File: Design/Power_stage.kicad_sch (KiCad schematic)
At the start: 25 parts, among them IC4 LM60440ARPKR, U3 CRE1S0505S3C, U6 CRE1S0505S3C, U8 LP3963-3.3

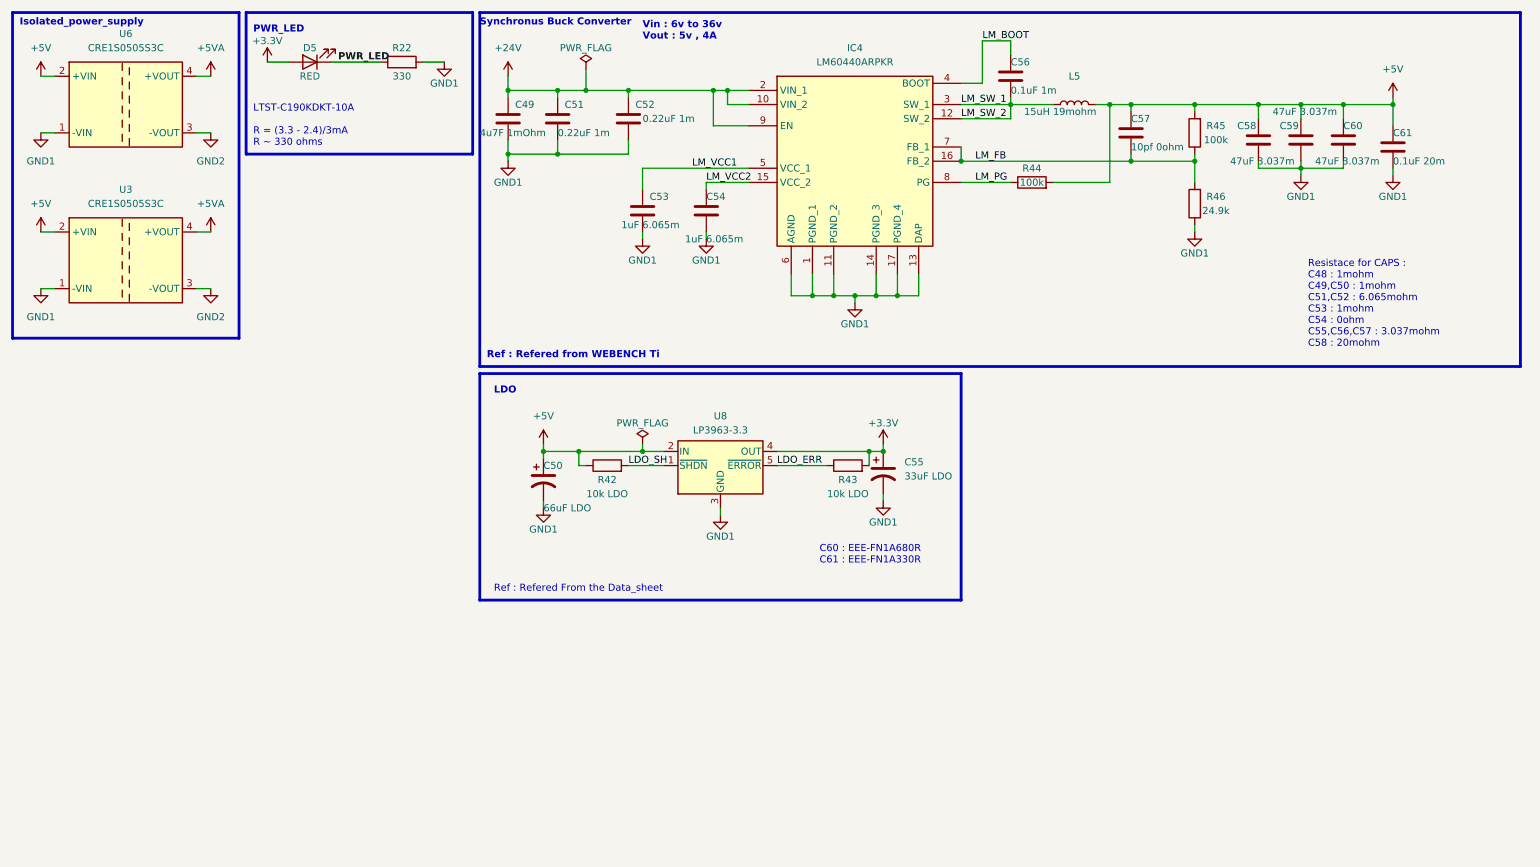
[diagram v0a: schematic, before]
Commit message: Schematic Design complete
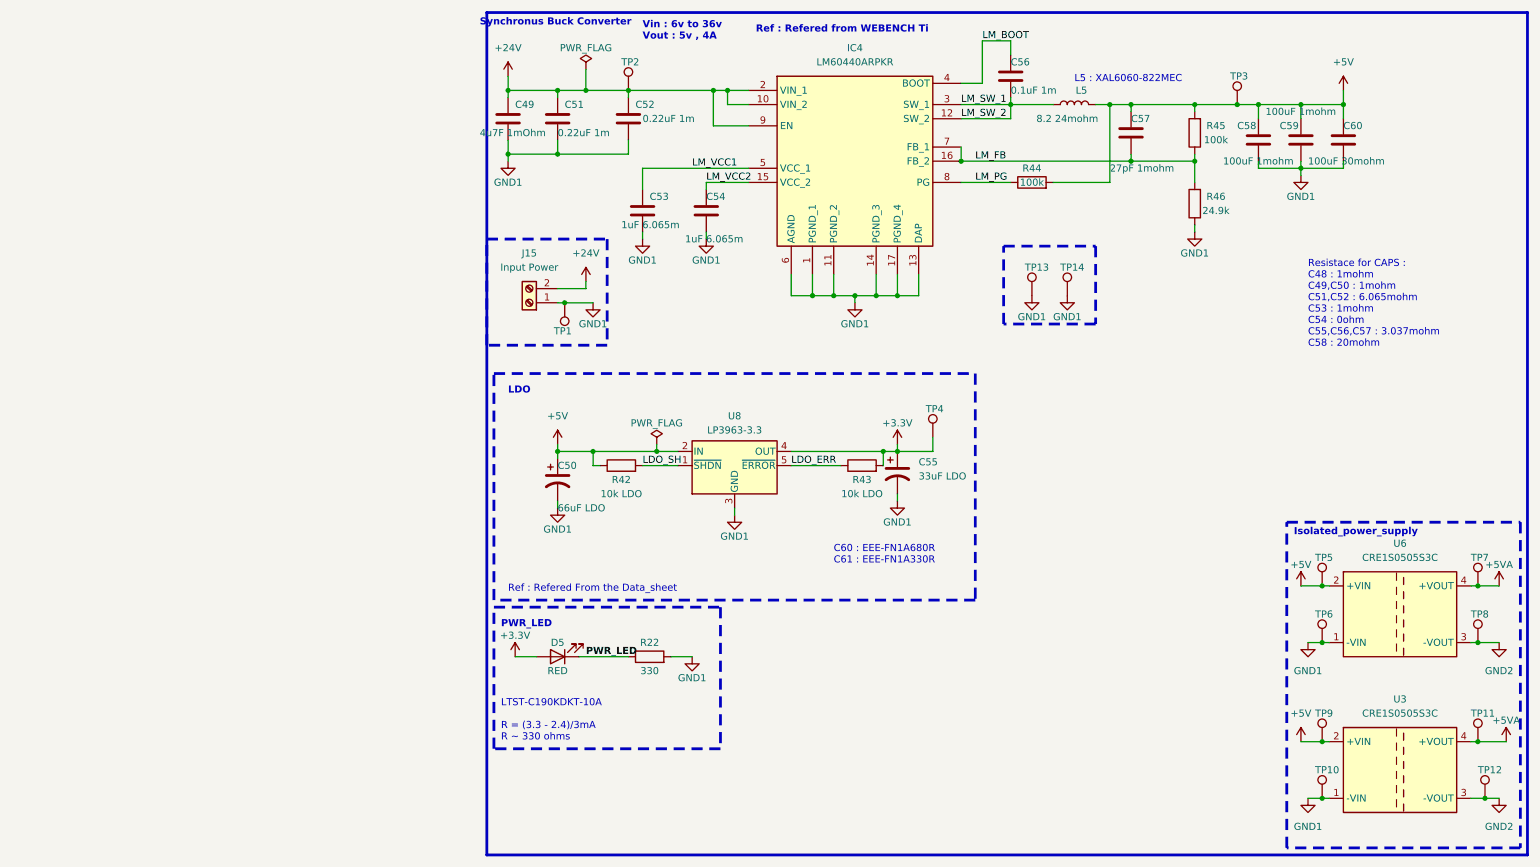
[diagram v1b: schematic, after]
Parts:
- removed C61: 0.1uF 20m, Capacitor_SMD:C_0603_1608Metric_Pad1.08x0.95mm_HandSolder, symbol Device:C
- added J15: Input Power, TerminalBlock_Phoenix:TerminalBlock_Phoenix_MKDS-1,5-2_1x02_P5.00mm_Horizontal, symbol Connector:Screw_Terminal_01x02
- added TP1, TP10, TP11, TP12, TP13, TP14, TP2, TP3, TP4, TP5, TP6, TP7, TP8, TP9: TestPoint, TestPoint:TestPoint_Pad_D2.5mm, symbol Connector:TestPoint
- C57: value 10pf 0ohm -> 27pF 1mohm
- C58, C59: value 47uF 3.037m -> 100uF 1mohm
- C60: value 47uF 3.037m -> 100uF 30mohm
- L5: value 15uH 19mohm -> 8.2 24mohm; footprint (none) -> Inductor_SMD:L_Coilcraft_XAL6060-XXX
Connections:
- net +24V: now also J15.2 (Pin_2), TP2.1
- net +3.3V: now also TP4.1
- net +5V: now also TP3.1, TP5.1, TP9.1
- net +5VA: now also TP11.1, TP7.1
- net GND1: now also J15.1 (Pin_1), TP1.1, TP10.1, TP13.1, TP14.1, TP6.1
- net GND2: now also TP12.1, TP8.1
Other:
- note added: "L5 : XAL6060-822MEC"
- moved on the sheet: C50, C55, D5, R22, R42, R43, U3, U6, U8
